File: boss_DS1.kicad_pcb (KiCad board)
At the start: 2 copper layers, 80 x 100 mm, 84 parts, among them J1 NMJ6HHD2, J2 NMJ6HHD2, J3 Conn_01x05, J4 Conn_01x05, J5 Conn_01x05, J6 Barrel_Jack_MountingPin, P1 boss_DS1_front_panel, Q1 MMBT5551, Q2 MMBT5551, Q3 MMBT5551, Q4 MMBT5551, SW1 pedala_switch, U1 NE5532

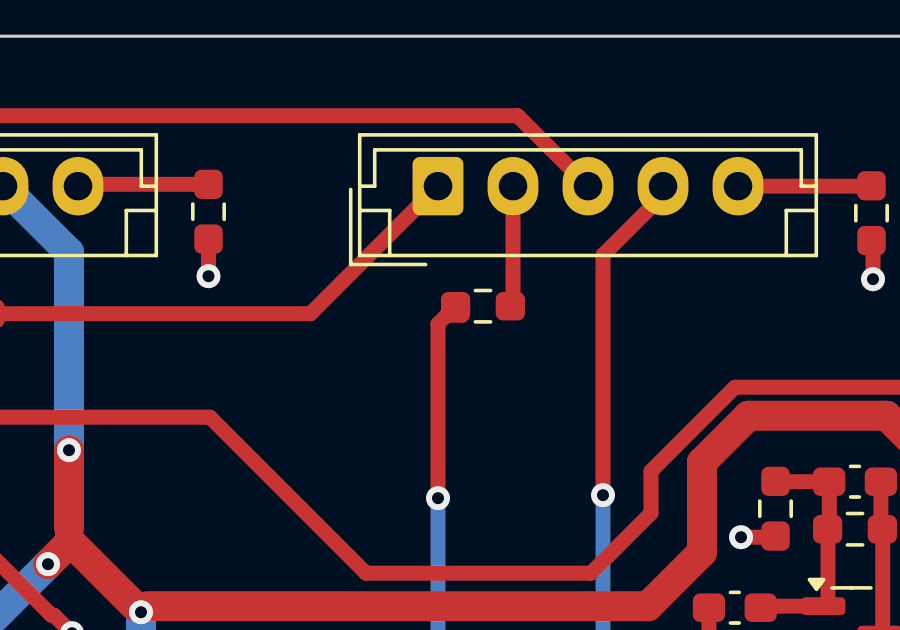
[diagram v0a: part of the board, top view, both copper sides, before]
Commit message: a
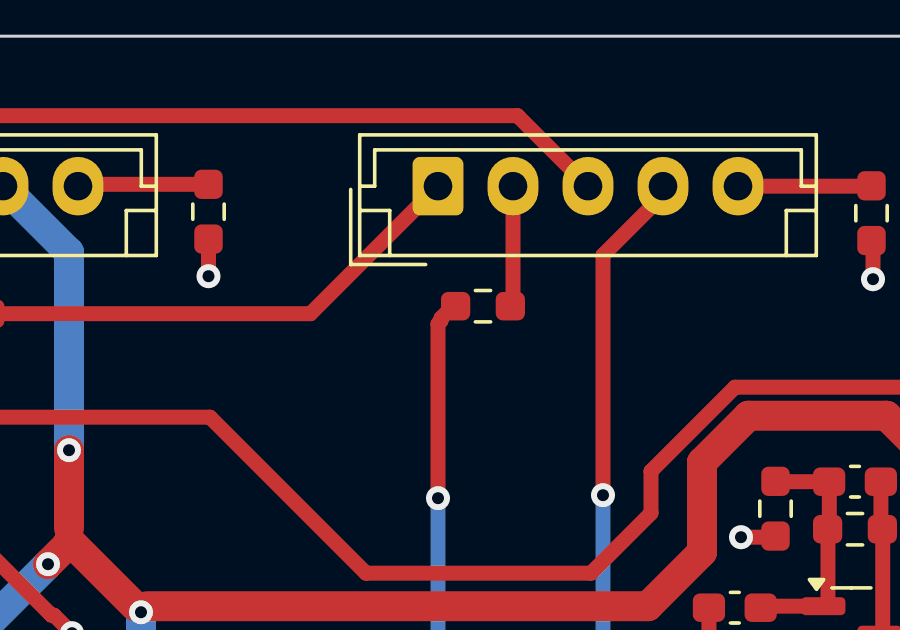
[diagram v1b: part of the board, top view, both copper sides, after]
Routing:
- net /SW_ON: track 64.2 -> 63.7 mm
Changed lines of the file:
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@@
 	)
 	(segment
-		(start 85.5 59)
-		(end 85.5875 59)
+		(start 85 59.5875)
+		(end 85.1 59.4875)
 		(width 0.5)
 		(layer "F.Cu")
@@
 	)
 	(segment
-		(start 85.2875 59.3)
-		(end 85.8 59.3)
+		(start 85 71.4)
+		(end 85 77.25)
+		(width 0.5)
+		(layer "F.Cu")
+		(net 25)
+	)
+	(segment
+		(start 85.1 59.4)
+		(end 85.5 59)
+		(width 0.5)
+		(layer "F.Cu")
+		(net 25)
+	)
+	(segment
+		(start 85.5 59)
+		(end 85.5875 59)
 		(width 0.5)
 		(layer "F.Cu")
@@
 	)
 	(segment
-		(start 85 71.4)
-		(end 85 77.25)
+		(start 85.1 59.4875)
+		(end 85.1 59.4)
 		(width 0.5)
 		(layer "F.Cu")
-		(net 25)
-	)
-	(segment
-		(start 85.8 59.3)
-		(end 85.5 59)
-		(width 0.5)
-		(layer "F.Cu")
-		(net 25)
-	)
-	(segment
-		(start 85 59.5875)
-		(end 85.2875 59.3)
-		(width 0.5)
-		(layer "F.Cu")
